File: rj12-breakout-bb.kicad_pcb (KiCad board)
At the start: 2 copper layers, 32.3 x 14.6 mm, 4 parts, among them J1 RJ12, J2 Front, J3 Back

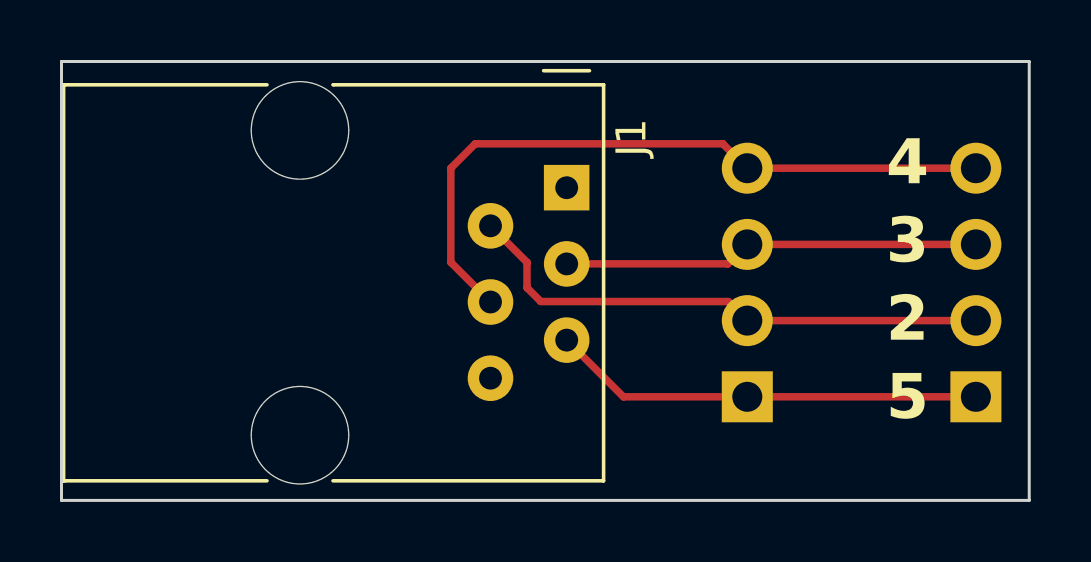
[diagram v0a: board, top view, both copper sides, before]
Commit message: Ordered Version 1.0
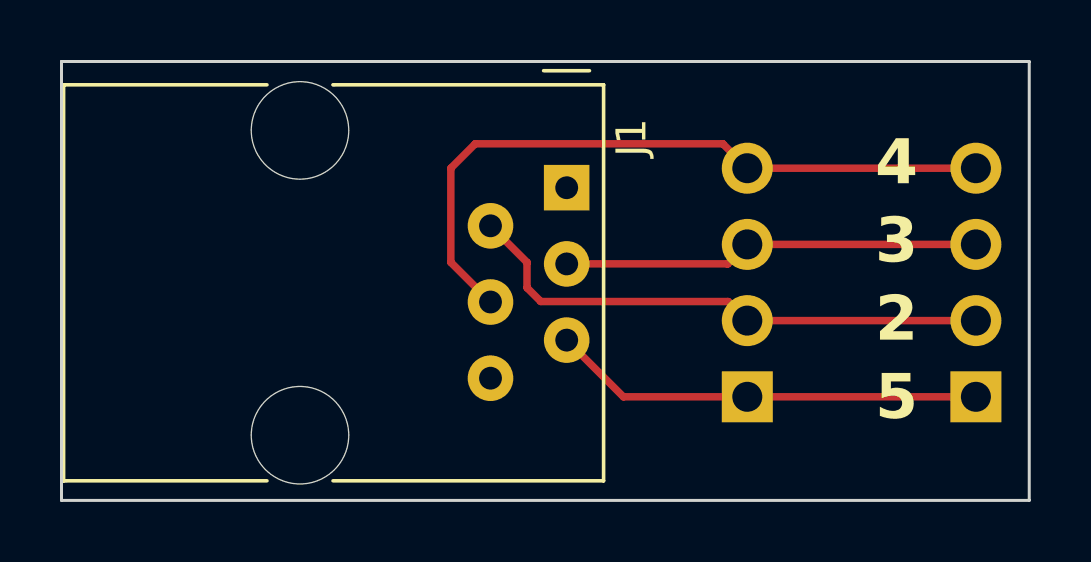
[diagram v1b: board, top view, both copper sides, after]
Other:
- board text added: "1"
- board text added: "6"
- board text added: "RJ12 BB v1.0 2023"
- board text removed: "RJ12 BB v1.1 2023"
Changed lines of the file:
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@@
   (gr_rect (start 93.98 69.723) (end 126.238 84.3534)
     (stroke (width 0.1) (type default)) (fill none) (layer "Edge.Cuts"))
-  (gr_text "RJ12 BB\nv1.1 2023" (at 107.0102 78.2066) (layer "B.SilkS")
+  (gr_text "RJ12 BB\nv1.0 2023" (at 106.8 77.4) (layer "B.SilkS")
     (effects (font (size 1 1) (thickness 0.15)) (justify left bottom mirror))
   )
-  (gr_text "5" (at 121.4628 81.788) (layer "F.SilkS")
+  (gr_text "2" (at 113.1 75.8) (layer "B.SilkS")
+    (effects (font (size 1 1) (thickness 0.15)) (justify left bottom mirror))
+  )
+  (gr_text "1" (at 114.5 74.6) (layer "B.SilkS")
+    (effects (font (size 1 1) (thickness 0.15)) (justify left bottom mirror))
+  )
+  (gr_text "5" (at 114.5 79.6) (layer "B.SilkS")
+    (effects (font (size 1 1) (thickness 0.15)) (justify left bottom mirror))
+  )
+  (gr_text "3" (at 114.5 77.1) (layer "B.SilkS")
+    (effects (font (size 1 1) (thickness 0.15)) (justify left bottom mirror))
+  )
+  (gr_text "6" (at 113.2 81) (layer "B.SilkS")
+    (effects (font (size 1 1) (thickness 0.15)) (justify left bottom mirror))
+  )
+  (gr_text "4" (at 113.2 78.4) (layer "B.SilkS")
+    (effects (font (size 1 1) (thickness 0.15)) (justify left bottom mirror))
+  )
+  (gr_text "5" (at 121.1 81.788) (layer "F.SilkS")
     (effects (font (size 1.5 1.5) (thickness 0.3) bold) (justify left bottom))
   )
-  (gr_text "4" (at 121.4628 73.9648) (layer "F.SilkS")
+  (gr_text "4" (at 121.1 73.9648) (layer "F.SilkS")
     (effects (font (size 1.5 1.5) (thickness 0.3) bold) (justify left bottom))
   )
-  (gr_text "3" (at 121.4628 76.572533) (layer "F.SilkS")
+  (gr_text "3" (at 121.1 76.572533) (layer "F.SilkS")
     (effects (font (size 1.5 1.5) (thickness 0.3) bold) (justify left bottom))
   )
-  (gr_text "2" (at 121.4628 79.180266) (layer "F.SilkS")
+  (gr_text "2" (at 121.1 79.180266) (layer "F.SilkS")
     (effects (font (size 1.5 1.5) (thickness 0.3) bold) (justify left bottom))
   )
